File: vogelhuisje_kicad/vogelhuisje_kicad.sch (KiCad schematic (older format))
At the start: 0 parts

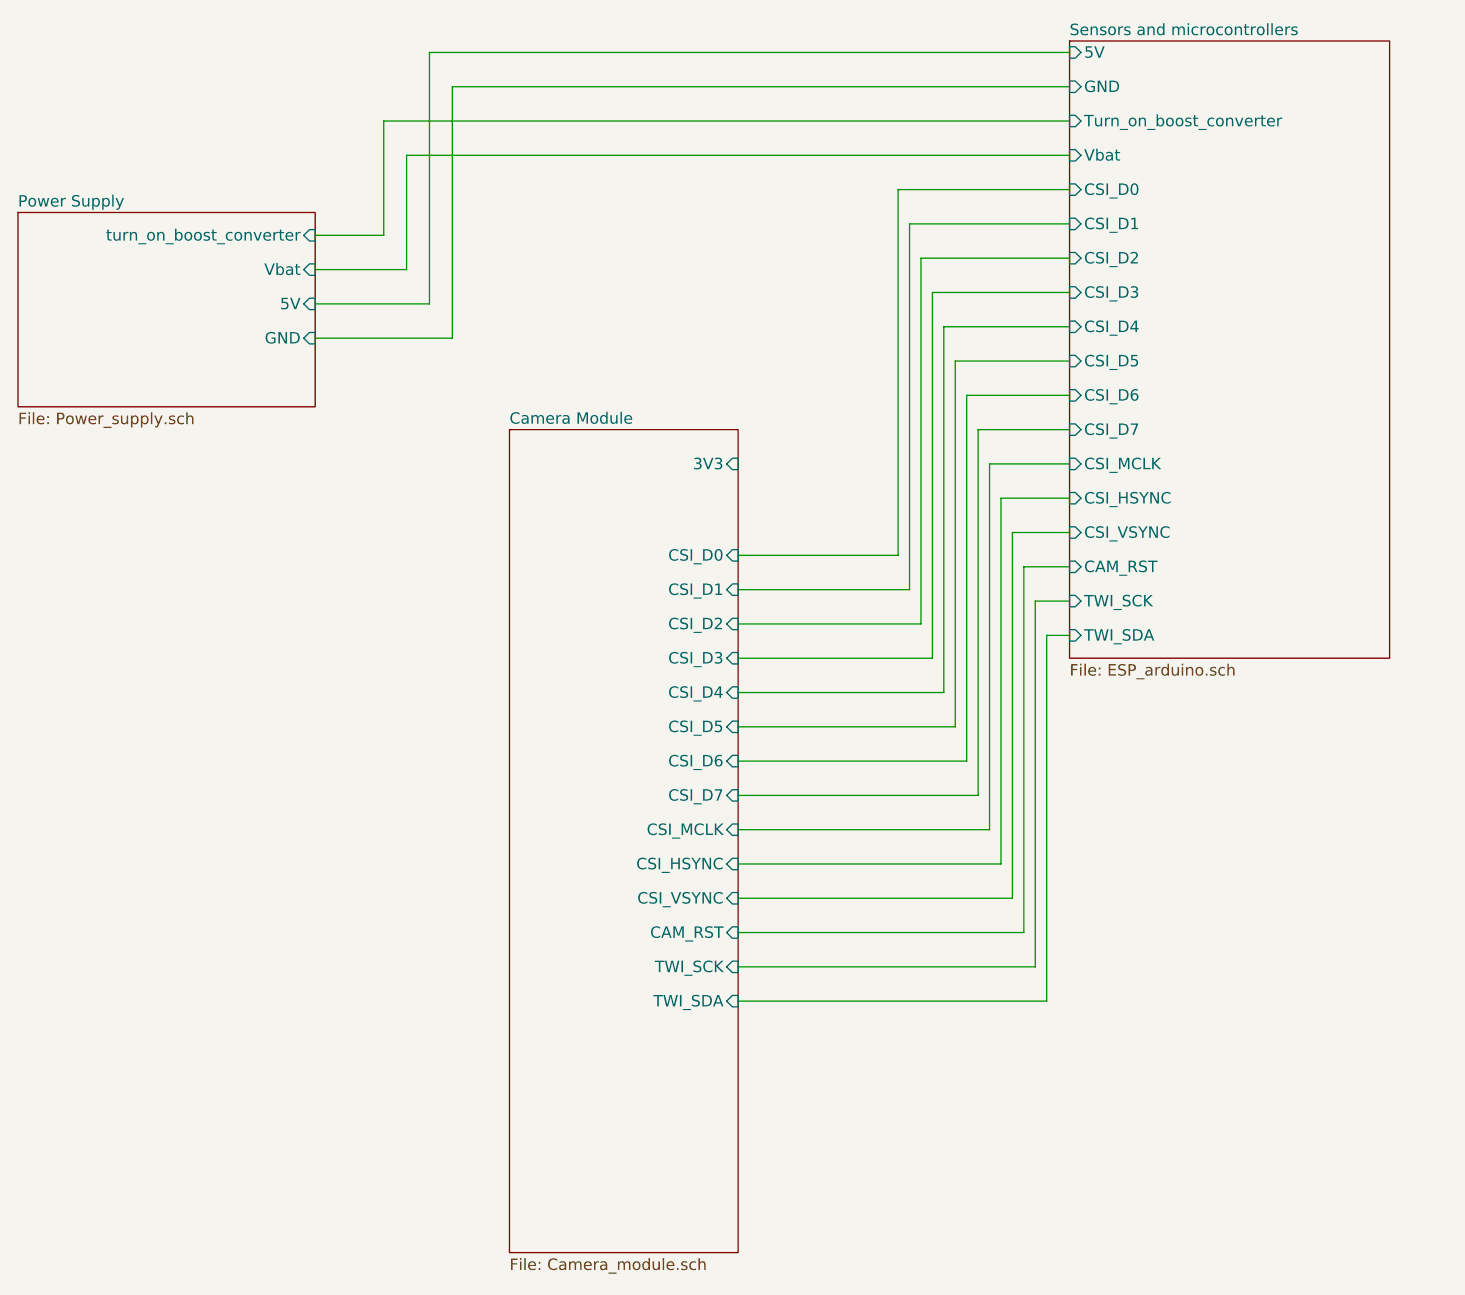
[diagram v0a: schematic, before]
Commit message: Update Camera_module.sch, Camera_module.sch-bak, and 5 more files...
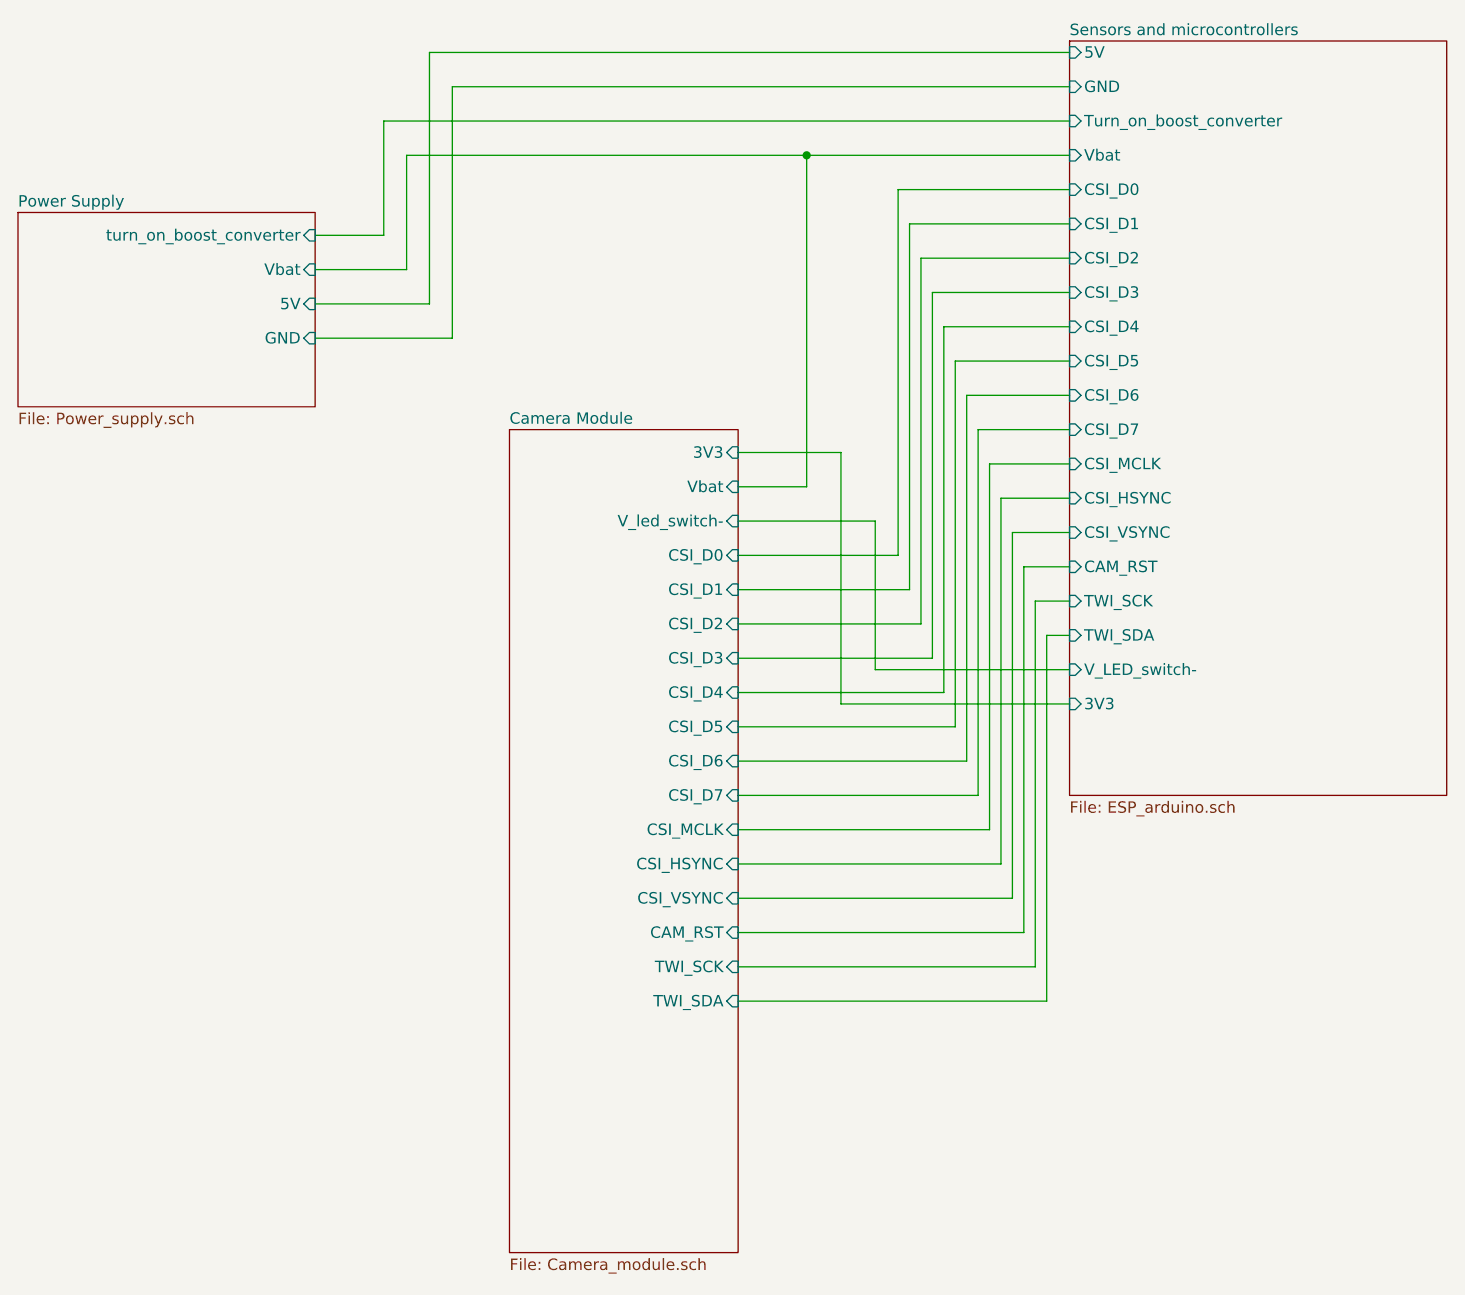
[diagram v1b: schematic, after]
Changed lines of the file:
@@
 $EndSheet
 $Sheet
-S 6300 1550 1400 2700
+S 6300 1550 1650 3300
 U 6263B902
 F0 "Sensors and microcontrollers" 50
@@
 F18 "Vbat" I L 6300 2050 50
 F19 "Turn_on_boost_converter" I L 6300 1900 50
+F20 "V_LED_switch-" I L 6300 4300 50
+F21 "3V3" I L 6300 4450 50
 $EndSheet
 Wire Wire Line
@@
 	3400 2550 3400 2050
 Wire Wire Line
-	3400 2050 6300 2050
+	3400 2050 5150 2050
 Wire Wire Line
 	3000 2700 3500 2700
@@
 Wire Wire Line
 	3600 1750 6300 1750
-$Sheet
-S 3850 3250 1000 3600
-U 626EFA13
-F0 "Camera Module" 50
-F1 "Camera_module.sch" 50
-F2 "CSI_D0" I R 4850 3800 50
-F3 "CSI_D1" I R 4850 3950 50
-F4 "CSI_D2" I R 4850 4100 50
-F5 "CSI_D3" I R 4850 4250 50
-F6 "CSI_D4" I R 4850 4400 50
-F7 "CSI_D5" I R 4850 4550 50
-F8 "CSI_D6" I R 4850 4700 50
-F9 "CSI_D7" I R 4850 4850 50
-F10 "CSI_MCLK" I R 4850 5000 50
-F11 "CSI_HSYNC" I R 4850 5150 50
-F12 "CSI_VSYNC" I R 4850 5300 50
-F13 "CAM_RST" I R 4850 5450 50
-F14 "TWI_SCK" I R 4850 5600 50
-F15 "TWI_SDA" I R 4850 5750 50
-F16 "3V3" I R 4850 3400 50
-$EndSheet
 Wire Wire Line
 	6300 4150 6200 4150
@@
 Wire Wire Line
 	5550 2200 6300 2200
+Wire Wire Line
+	6300 4450 5300 4450
+Wire Wire Line
+	5300 3350 4850 3350
+$Sheet
+S 3850 3250 1000 3600
+U 626EFA13
+F0 "Camera Module" 50
+F1 "Camera_module.sch" 50
+F2 "CSI_D0" I R 4850 3800 50
+F3 "CSI_D1" I R 4850 3950 50
+F4 "CSI_D2" I R 4850 4100 50
+F5 "CSI_D3" I R 4850 4250 50
+F6 "CSI_D4" I R 4850 4400 50
+F7 "CSI_D5" I R 4850 4550 50
+F8 "CSI_D6" I R 4850 4700 50
+F9 "CSI_D7" I R 4850 4850 50
+F10 "CSI_MCLK" I R 4850 5000 50
+F11 "CSI_HSYNC" I R 4850 5150 50
+F12 "CSI_VSYNC" I R 4850 5300 50
+F13 "CAM_RST" I R 4850 5450 50
+F14 "TWI_SCK" I R 4850 5600 50
+F15 "TWI_SDA" I R 4850 5750 50
+F16 "3V3" I R 4850 3350 50
+F17 "V_led_switch-" I R 4850 3650 50
+F18 "Vbat" I R 4850 3500 50
+$EndSheet
+Wire Wire Line
+	5300 3350 5300 4450
+Wire Wire Line
+	4850 3500 5150 3500
+Wire Wire Line
+	5150 3500 5150 2050
+Connection ~ 5150 2050
+Wire Wire Line
+	5150 2050 6300 2050
+Wire Wire Line
+	4850 3650 5450 3650
+Wire Wire Line
+	5450 3650 5450 4300
+Wire Wire Line
+	5450 4300 6300 4300
 $EndSCHEMATC
